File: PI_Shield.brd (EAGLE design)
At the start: 78.9 x 65.3 mm, 64 parts, among them Q1 220mA/50V/3.5Ω, Q3 220mA/50V/3.5Ω, Q4 220mA/50V/3.5Ω, Q5 2.5A/30V/105mΩ, U1 MAX1136EUA-T, U2 AZ1117EH-3.3TRG1, Y1 ECS-80-S-4X

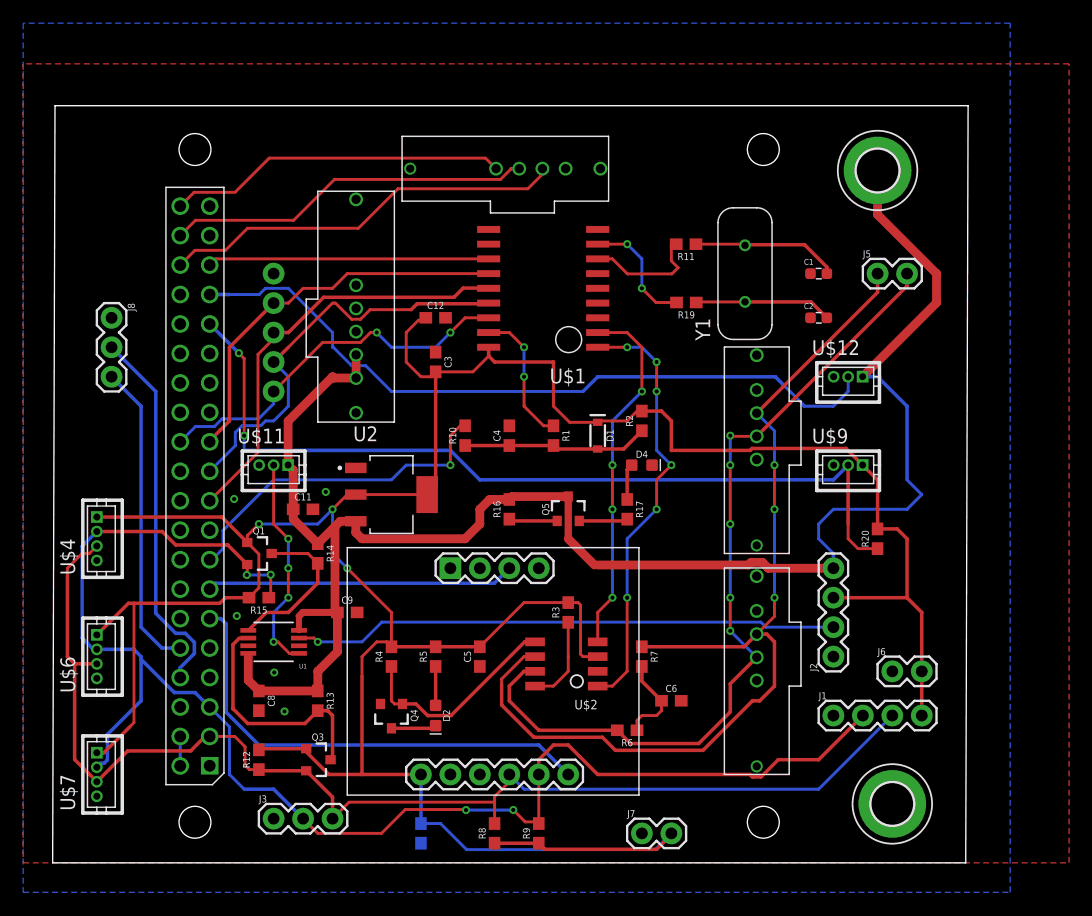
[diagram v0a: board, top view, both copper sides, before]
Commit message: Update PI_Shield.brd
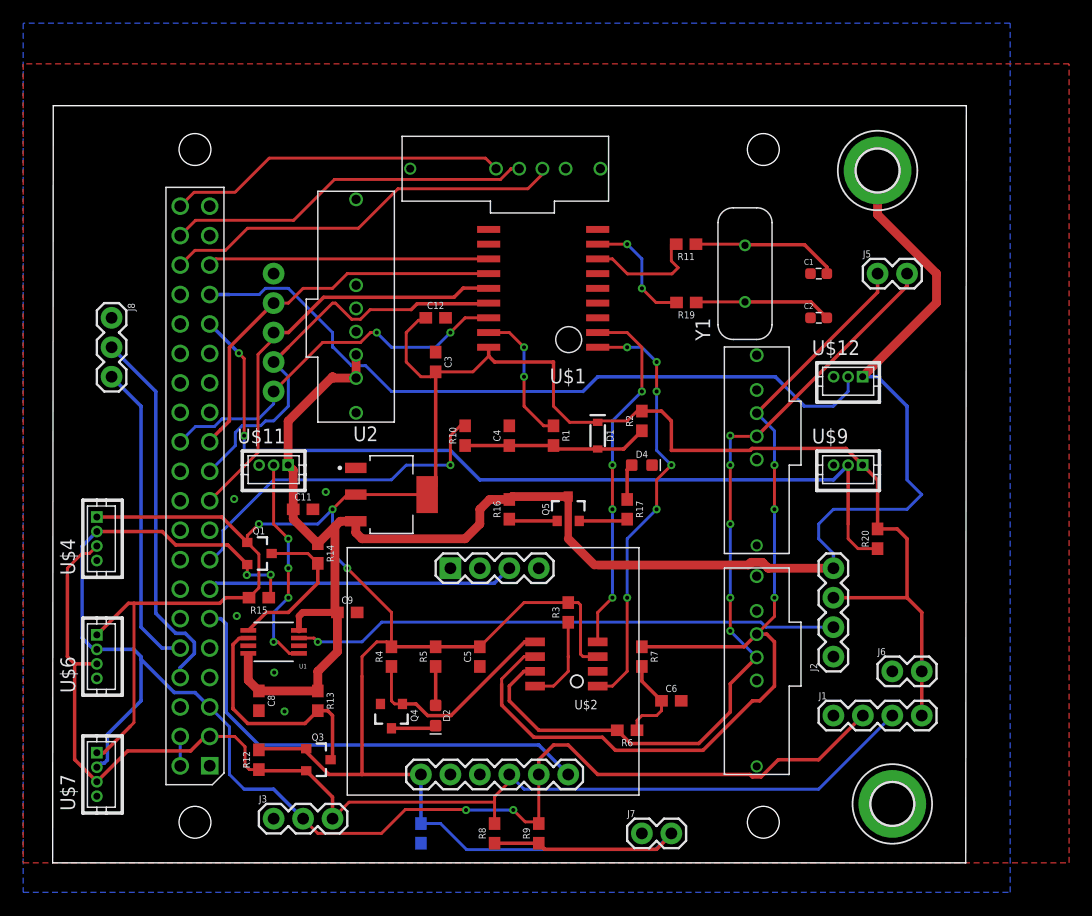
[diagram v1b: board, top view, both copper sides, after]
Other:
- board size 78.9 x 65.3 mm -> 78.8 x 65.3 mm
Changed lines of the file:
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@@
 <plain>
 <wire x1="13.97" y1="8.89" x2="92.69" y2="8.89" width="0" layer="20"/>
-<wire x1="92.69" y1="8.89" x2="92.8932" y2="74.1682" width="0" layer="20"/>
-<wire x1="92.8932" y1="74.1682" x2="14.1732" y2="74.1682" width="0" layer="20"/>
-<wire x1="14.1732" y1="74.1682" x2="13.97" y2="8.89" width="0" layer="20"/>
+<wire x1="92.69" y1="8.89" x2="92.7408" y2="74.1682" width="0" layer="20"/>
+<wire x1="92.7408" y1="74.1682" x2="14.0208" y2="74.1682" width="0" layer="20"/>
+<wire x1="14.0208" y1="74.1682" x2="13.97" y2="8.89" width="0" layer="20"/>
 </plain>
 <attributes>
